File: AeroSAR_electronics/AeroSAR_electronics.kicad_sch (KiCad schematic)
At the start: 3 parts, among them J1 USB_A

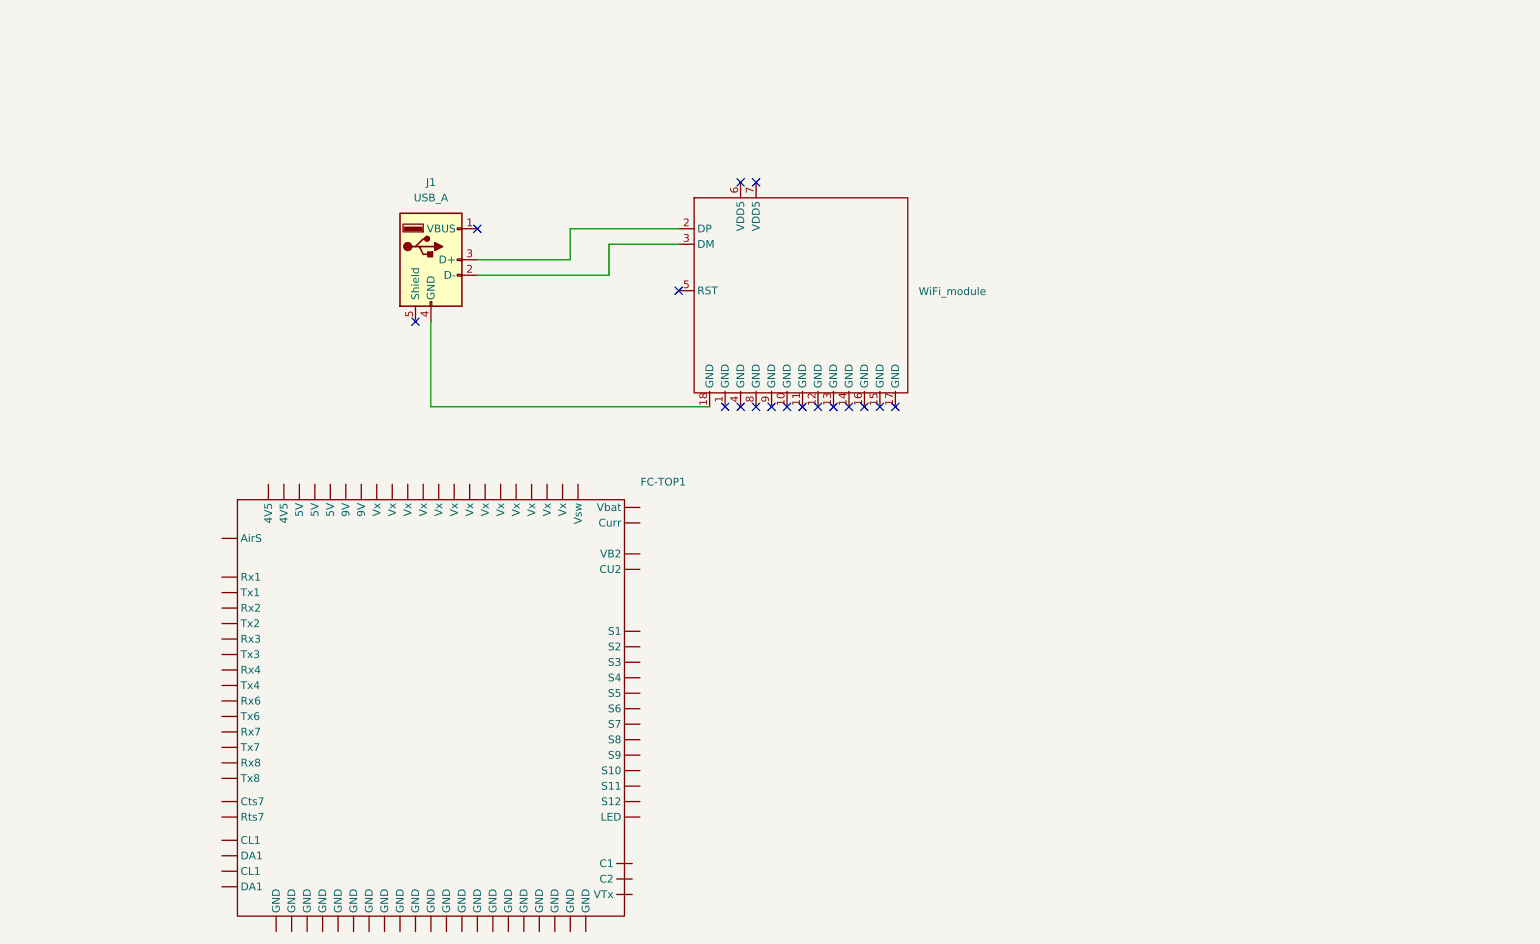
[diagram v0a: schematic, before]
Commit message: Prepared v1 of the schematic
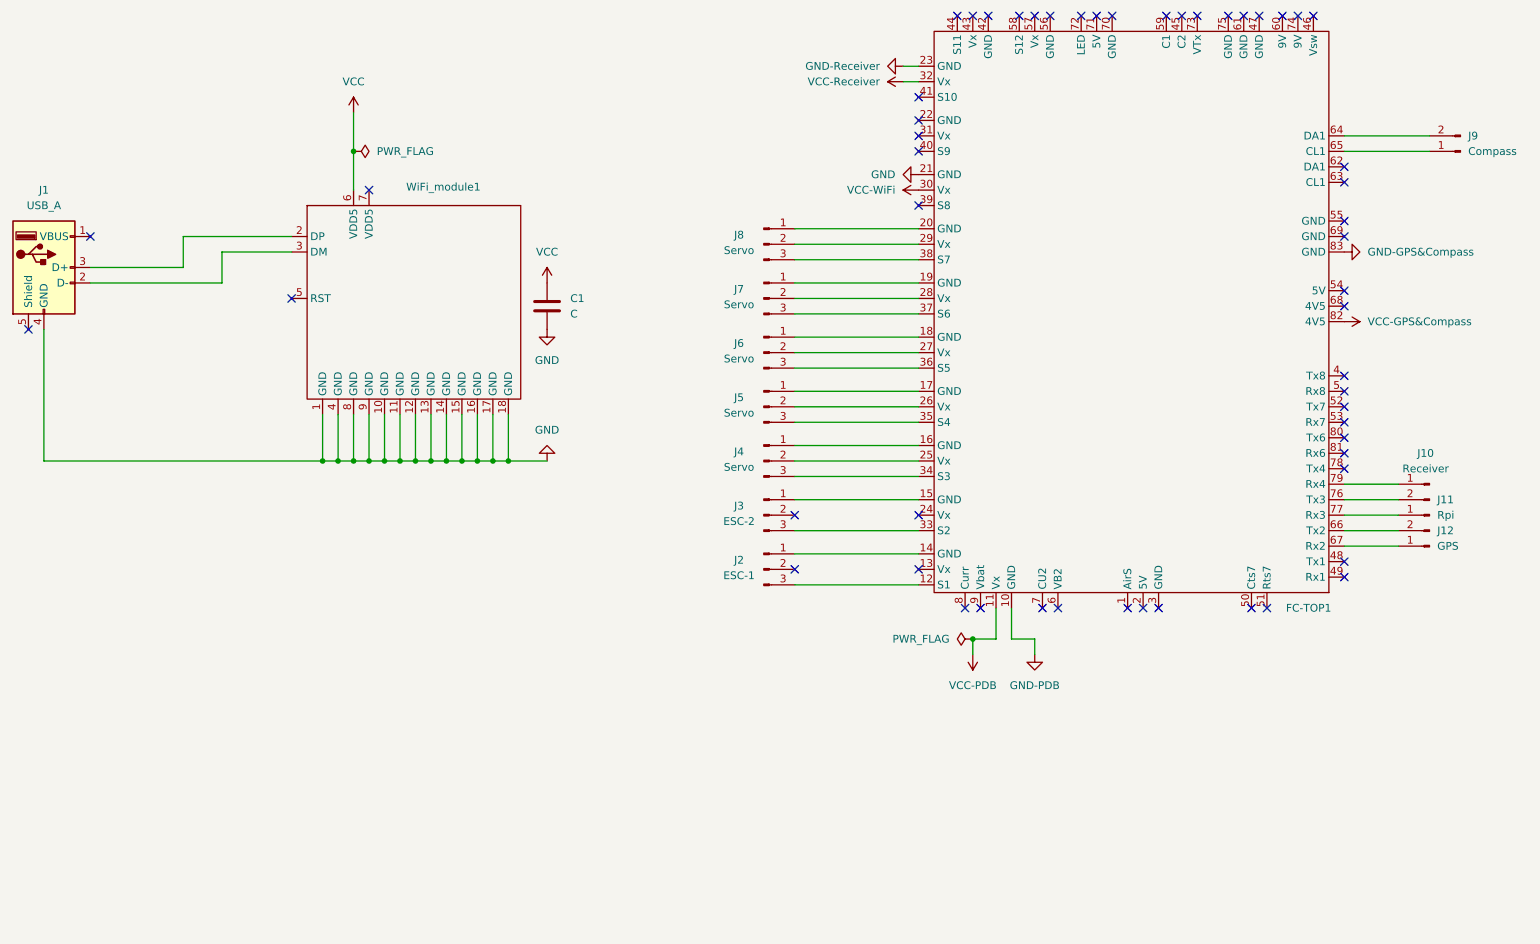
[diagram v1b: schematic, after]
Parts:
- removed WiFi_module: ~, BL-M8812EU2:BL-M8812EU2, symbol WiFi_module:BL-M8812EU2
- added C1: C, Capacitor_SMD:C_0805_2012Metric, symbol Device:C
- added J10: Receiver, symbol Connector:Conn_01x01_Pin
- added J11: Rpi, symbol Connector:Conn_01x02_Pin
- added J12: GPS, symbol Connector:Conn_01x02_Pin
- added J2: ESC-1, symbol Connector:Conn_01x03_Pin
- added J3: ESC-2, symbol Connector:Conn_01x03_Pin
- added J4, J5, J6, J7, J8: Servo, symbol Connector:Conn_01x03_Pin
- added J9: Compass, symbol Connector:Conn_01x02_Pin
- added WiFi_module1: ~, H743-WING-Top, symbol WiFi_module:BL-M8812EU2
- FC-TOP1: footprint (none) -> H743-WING-Top
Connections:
- net at J1.2 (D-): now also WiFi_module1.3 (DM)
- net at J1.3 (D+): now also WiFi_module1.2 (DP)
- net GND: now reaches J1.4 (GND)
- net GND: now also FC-TOP1.21 (GND), C1.2, WiFi_module1.1 (GND), WiFi_module1.10 (GND), WiFi_module1.11 (GND), WiFi_module1.12 (GND), WiFi_module1.13 (GND), WiFi_module1.14 (GND), WiFi_module1.15 (GND), WiFi_module1.16 (GND), WiFi_module1.17 (GND), WiFi_module1.18 (GND), WiFi_module1.4 (GND), WiFi_module1.8 (GND), WiFi_module1.9 (GND)
- new net: FC-TOP1.79 (Rx4), J10.1 (Pin_1)
- new net: FC-TOP1.18 (GND), J6.1 (Pin_1)
- new net: FC-TOP1.27 (Vx), J6.2 (Pin_2)
- new net: FC-TOP1.36 (S5), J6.3 (Pin_3)
- new net: FC-TOP1.14 (GND), J2.1 (Pin_1)
- new net: FC-TOP1.12 (S1), J2.3 (Pin_3)
- new net: FC-TOP1.15 (GND), J3.1 (Pin_1)
- new net: FC-TOP1.33 (S2), J3.3 (Pin_3)
- new net: FC-TOP1.67 (Rx2), J12.1 (Pin_1)
- new net: FC-TOP1.66 (Tx2), J12.2 (Pin_2)
- new net: FC-TOP1.65 (CL1), J9.1 (Pin_1)
- new net: FC-TOP1.64 (DA1), J9.2 (Pin_2)
- new net: FC-TOP1.77 (Rx3), J11.1 (Pin_1)
- new net: FC-TOP1.76 (Tx3), J11.2 (Pin_2)
- new net: FC-TOP1.20 (GND), J8.1 (Pin_1)
- new net: FC-TOP1.29 (Vx), J8.2 (Pin_2)
- new net: FC-TOP1.38 (S7), J8.3 (Pin_3)
- new net: FC-TOP1.19 (GND), J7.1 (Pin_1)
- new net: FC-TOP1.28 (Vx), J7.2 (Pin_2)
- new net: FC-TOP1.37 (S6), J7.3 (Pin_3)
- new net: FC-TOP1.17 (GND), J5.1 (Pin_1)
- new net: FC-TOP1.26 (Vx), J5.2 (Pin_2)
- new net: FC-TOP1.35 (S4), J5.3 (Pin_3)
- new net: FC-TOP1.16 (GND), J4.1 (Pin_1)
- new net: FC-TOP1.25 (Vx), J4.2 (Pin_2)
- new net: FC-TOP1.34 (S3), J4.3 (Pin_3)
- new net GND-GPS&Compass: FC-TOP1.83 (GND)
- new net GND-PDB: FC-TOP1.10 (GND)
- new net GND-Receiver: FC-TOP1.23 (GND)
- new net VCC: C1.1, WiFi_module1.6 (VDD5)
- new net VCC-GPS&Compass: FC-TOP1.82 (4V5)
- new net VCC-PDB: FC-TOP1.11 (Vx)
- new net VCC-Receiver: FC-TOP1.32 (Vx)
- new net VCC-WiFi: FC-TOP1.30 (Vx)
- no-connect marks 17 -> 55
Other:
- moved on the sheet: J1
